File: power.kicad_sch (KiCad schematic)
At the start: 66 parts, among them J5 S7B-XH-A

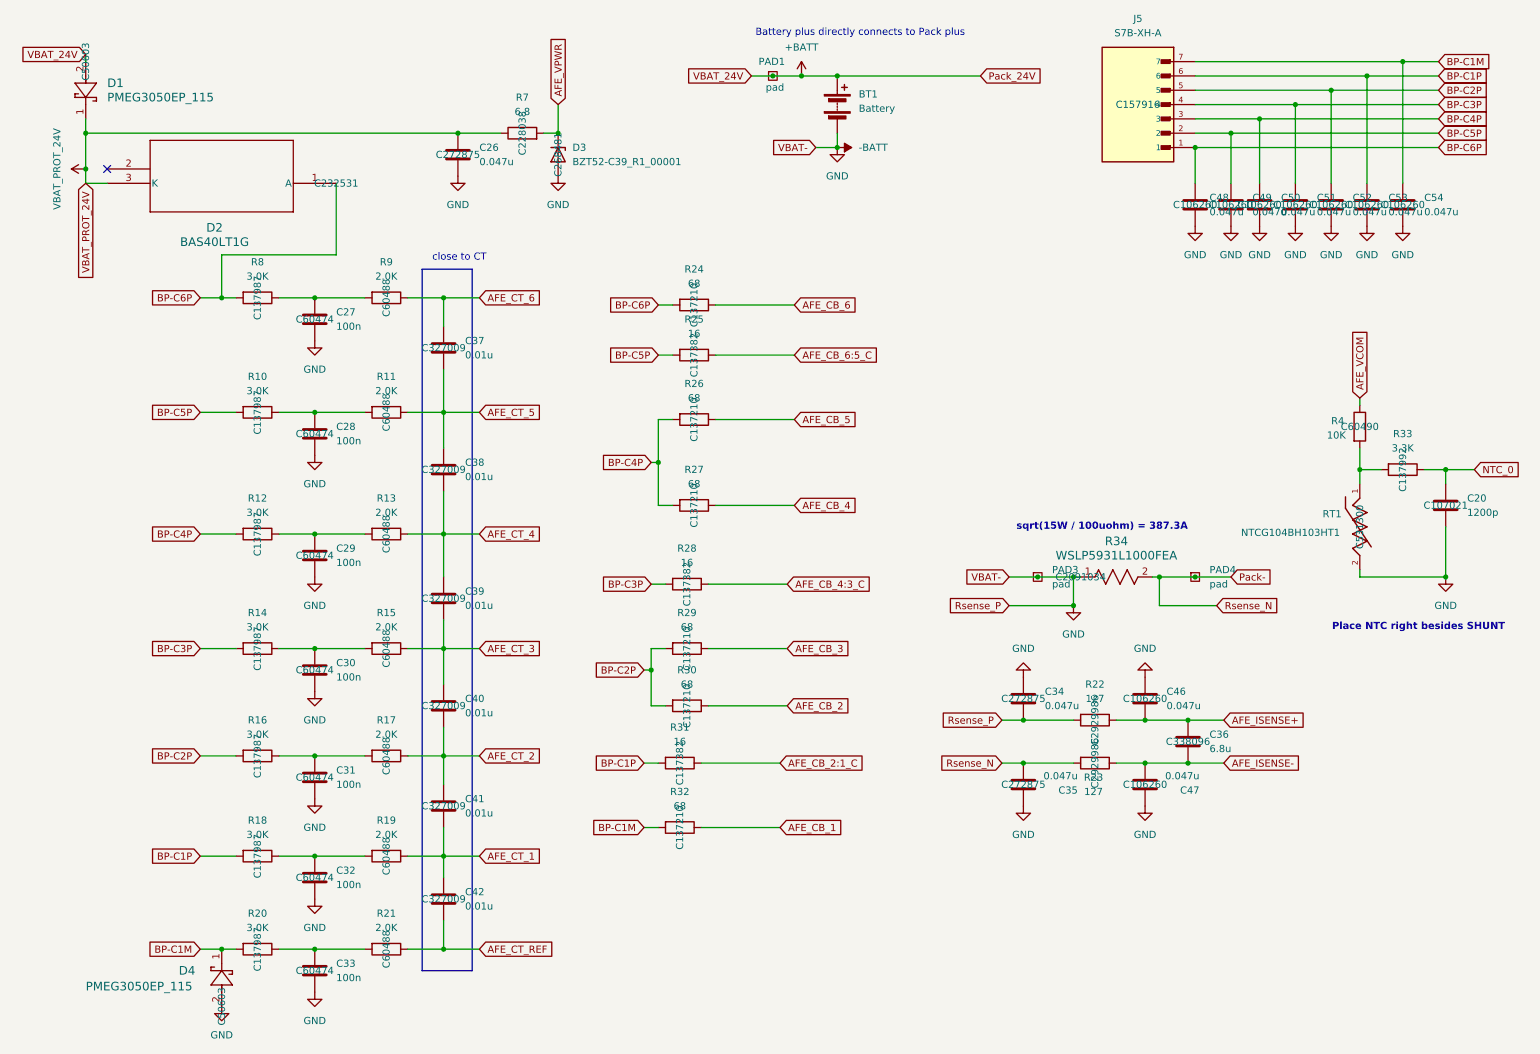
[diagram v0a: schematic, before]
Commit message: for PCBWay
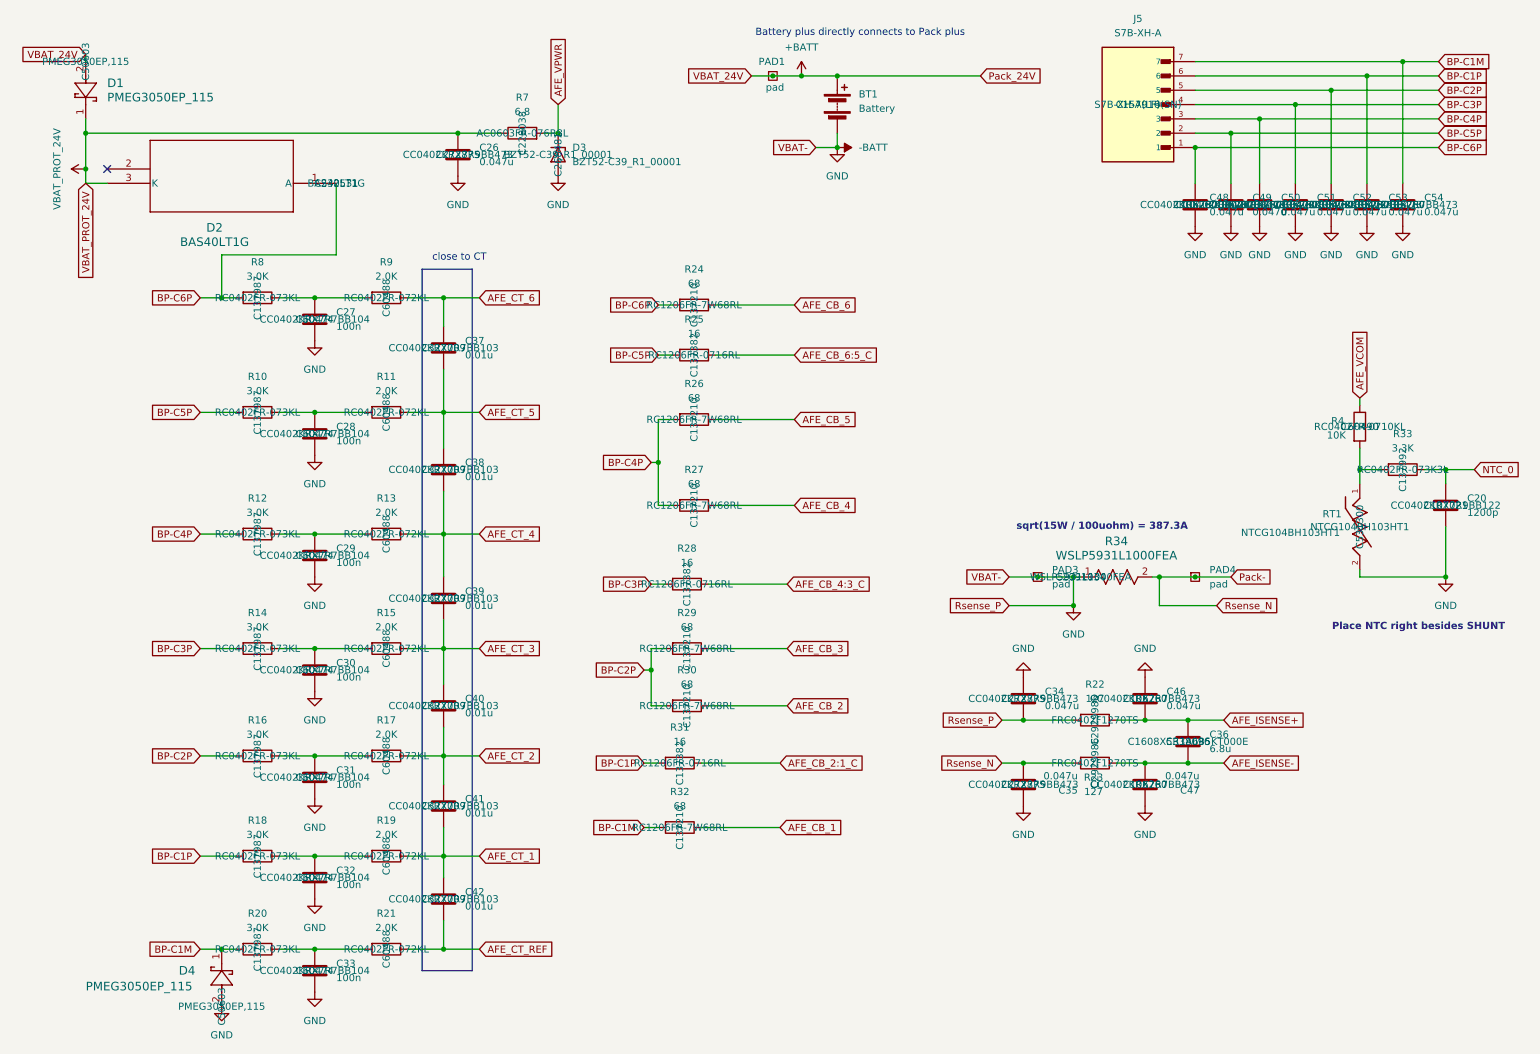
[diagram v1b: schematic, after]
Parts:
- C20: MPN (none) -> CC0402KRX7R9BB122
- C26, C34, C35: MPN (none) -> CC0402KRX7R9BB473
- C27, C28, C29, C30, C31, C32, C33: MPN (none) -> CC0402KRX7R7BB104
- C36: MPN (none) -> C1608X5R1A685KT000E
- C37, C38, C39, C40, C41, C42: MPN (none) -> CC0402KRX7R7BB103
- C46, C47, C48, C49, C50, C51, C52, C53, C54: MPN (none) -> CC0402KRX7R7BB473
- D1, D4: MPN (none) -> PMEG3050EP,115
- D2: MPN (none) -> BAS40LT1G
- D3: MPN (none) -> BZT52-C39_R1_00001
- J5: MPN (none) -> S7B-XH-A(LF)(SN)
- R10, R12, R14, R16, R18, R20, R8: MPN (none) -> RC0402FR-073KL
- R11, R13, R15, R17, R19, R21, R9: MPN (none) -> RC0402FR-072KL
- R22, R23: MPN (none) -> FRC0402F1270TS
- R24, R26, R27, R29, R30, R32: MPN (none) -> RC1206FR-7W68RL
- R25, R28, R31: MPN (none) -> RC1206FR-0716RL
- R33: MPN (none) -> RC0402FR-073K3L
- R34: MPN (none) -> WSLP5931L1000FEA
- R4: MPN (none) -> RC0402FR-0710KL
- R7: MPN (none) -> AC0603FR-076R8L
- RT1: MPN (none) -> NTCG104BH103HT1
